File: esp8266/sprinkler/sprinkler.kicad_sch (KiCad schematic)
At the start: 27 parts, among them Q1 AO4407A, U1 MAX1873TEEE

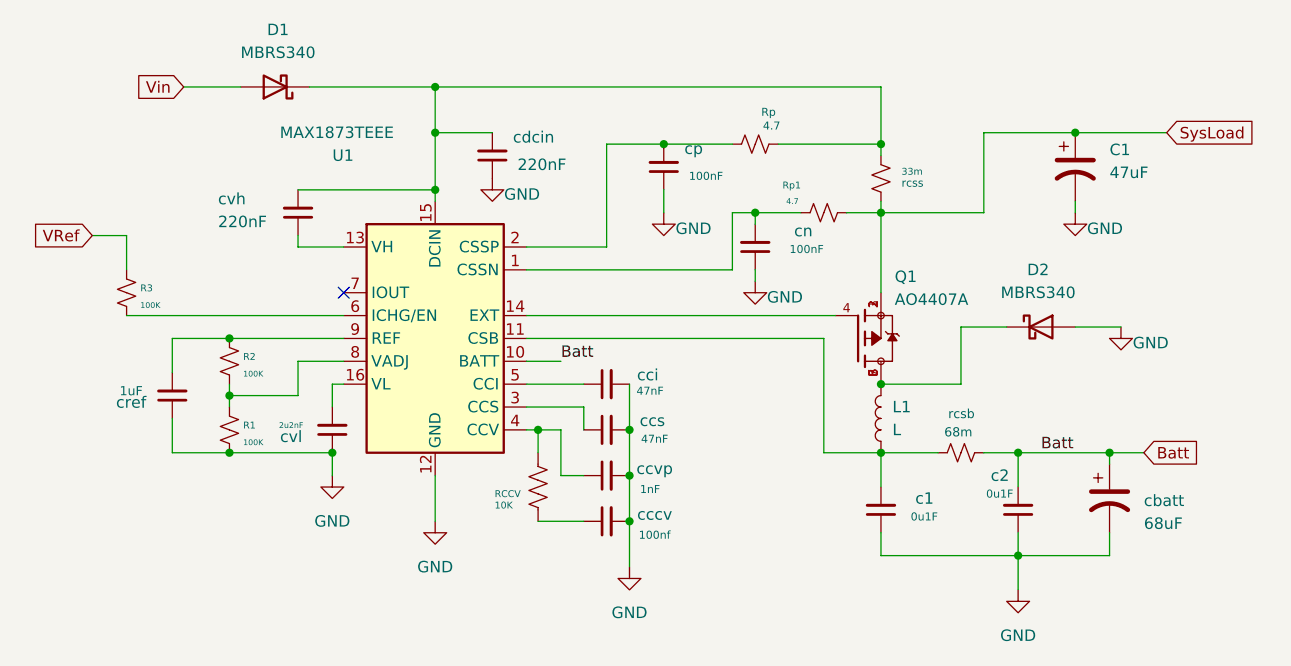
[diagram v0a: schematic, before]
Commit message: New sheets
Added power sheet and micro controller sheet
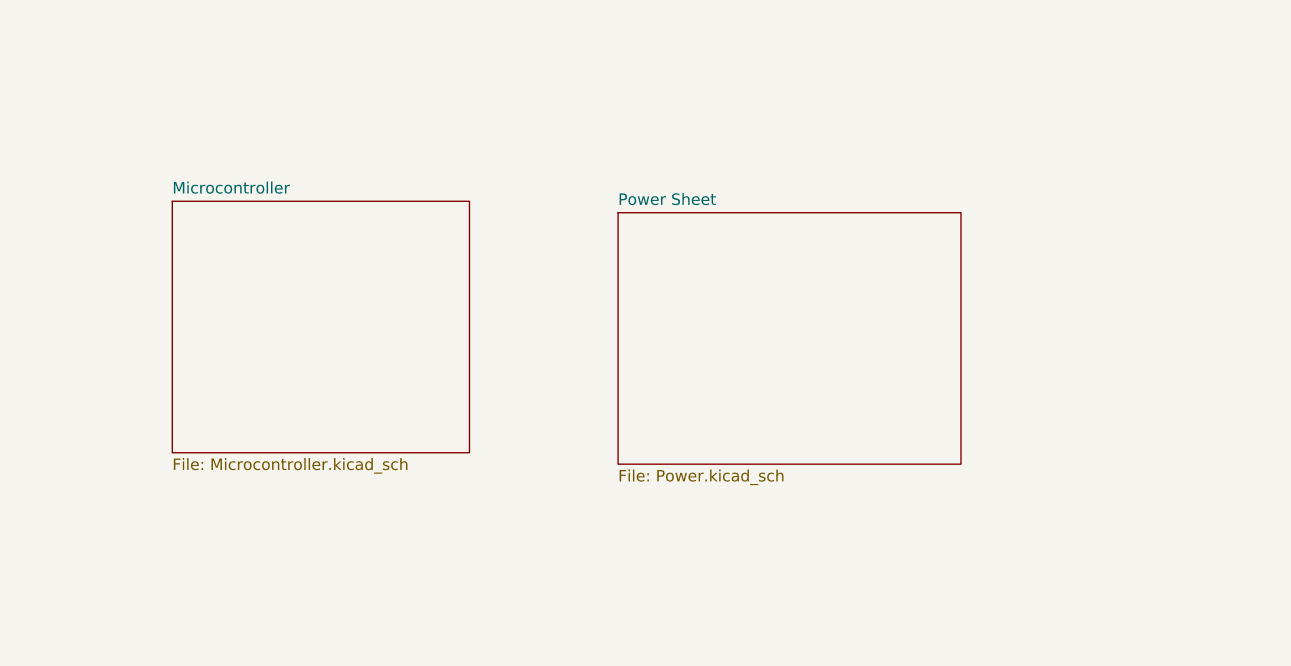
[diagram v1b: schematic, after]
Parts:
- removed C1: 47uF, symbol Device:C_Polarized_US
- removed D1, D2: MBRS340, Diode_SMD:D_SMC, symbol Diode:MBRS340
- removed L1: L, symbol Device:L
- removed Q1: AO4407A, AO4407A:SOIC127P600X175-8N, symbol Alpha_Omega:AO4407A
- removed R1, R2, R3: 100K, symbol Device:R_Small_US
- removed RCCV: 10K, symbol Device:R_US
- removed Rp, Rp1: 4.7, symbol Device:R_Small_US
- removed U1: MAX1873TEEE, Package_SO:QSOP-16_3.9x4.9mm_P0.635mm, symbol Battery_Management:MAX1873TEEE
- removed c1, c2: 0u1F, symbol Device:C_Small
- removed cbatt: 68uF, symbol Device:C_Polarized_US
- removed cccv: 100nf, symbol Device:C_Small
- removed cci, ccs: 47nF, symbol Device:C_Small
- removed ccvp: 1nF, symbol Device:C_Small
- removed cdcin, cvh: 220nF, symbol Device:C_Small
- removed cn, cp: 100nF, symbol Device:C_Small
- removed cref: 1uF, symbol Device:C_Small
- removed cvl: 2u2nF, symbol Device:C_Small
- removed rcsb: 68m, symbol Device:R_Small_US
- removed rcss: 33m, symbol Device:R_Small_US
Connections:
- no-connect marks 1 -> 0
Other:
- added sheet Microcontroller (Microcontroller.kicad_sch)
- added sheet Power Sheet (Power.kicad_sch)
